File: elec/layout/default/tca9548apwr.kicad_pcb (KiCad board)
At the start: 2 copper layers, 20 parts

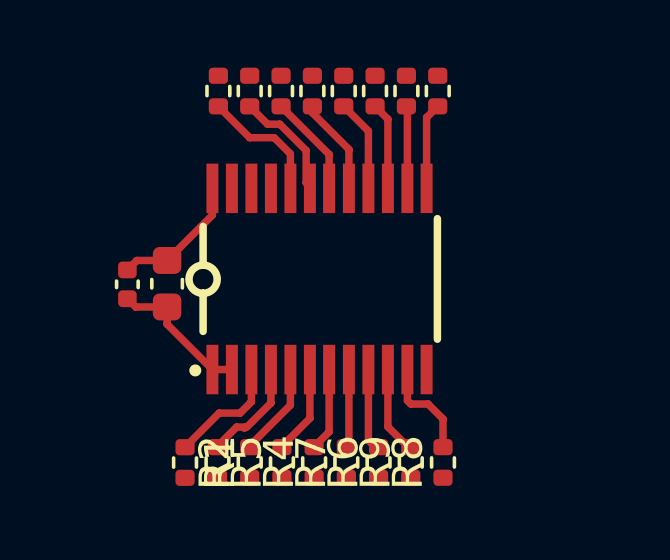
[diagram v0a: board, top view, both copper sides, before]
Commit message: run build, update layout
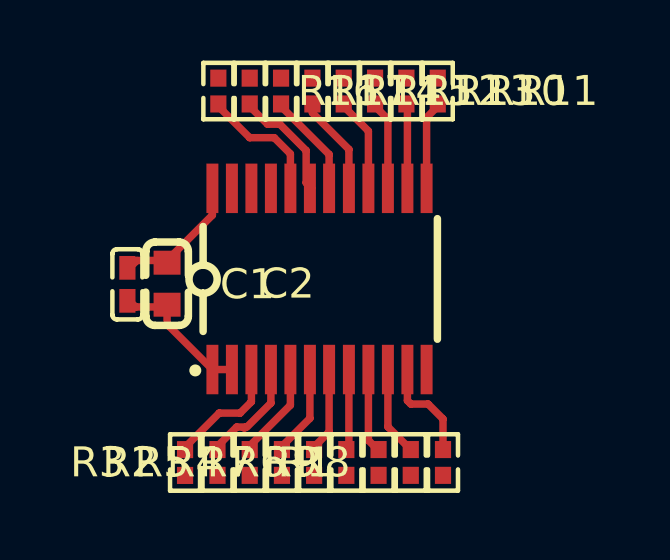
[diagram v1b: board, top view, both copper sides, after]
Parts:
- C1: value 16V 100nF X7R ±10% 0402 Multilayer Ceramic Capacitors MLCC - SMD/SMT ROHS -> 100nF ±10% 16V X7R; footprint lib:C0402 -> lcsc:C0402
- C2: value 16V 2.2uF X5R ±10% 0603 Multilayer Ceramic Capacitors MLCC - SMD/SMT ROHS -> 2.2µF ±10% 25V X5R; footprint lib:C0603 -> lcsc:C0603
- R1, R10, R11, R12, R13, R14, R15, R16, R17, R2, R3, R4, R5, R6, R7, R8, R9: value 62.5mW Thick Film Resistors 50V ±100ppm/℃ ±1% 10kΩ 0402 Chip Resistor - Surface Mount ROHS -> 10kΩ ±1% 62.5mW; footprint lib:R0402 -> lcsc:R0402
- U1: value (none) -> _TCA9548APWR
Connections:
- net ic-gnd renamed gnd
- net ic-scl renamed scl-5
- net ic-scl-1 renamed scl
- net ic-scl-2 renamed scl-2
- net ic-scl-3 renamed scl-6
- net ic-scl-4 renamed scl-3
- net ic-scl-5 renamed scl-4
- net ic-scl-6 renamed scl-7
- net ic-scl-7 renamed scl-1
- net ic-scl-8 renamed SCL
- net ic-sda renamed sda-5
- net ic-sda-1 renamed sda-7
- net ic-sda-2 renamed sda-3
- net ic-sda-3 renamed sda-6
- net ic-sda-4 renamed sda-4
- net ic-sda-5 renamed sda
- net ic-sda-6 renamed sda-2
- net ic-sda-7 renamed sda-1
- net ic-sda-8 renamed SDA
- net reset_ renamed io
- net vcc renamed hv
